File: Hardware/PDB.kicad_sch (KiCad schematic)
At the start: 52 parts, among them J1 Conn_01x02, J2 Conn_01x02, J3 Conn_01x02, J4 Conn_01x02, J5 Conn_01x02, Q1 Q_PMOS_GDS, U1 TPS54302, U2 TPS54302, U3 AP2112K-1.8, U4 INA219AxD

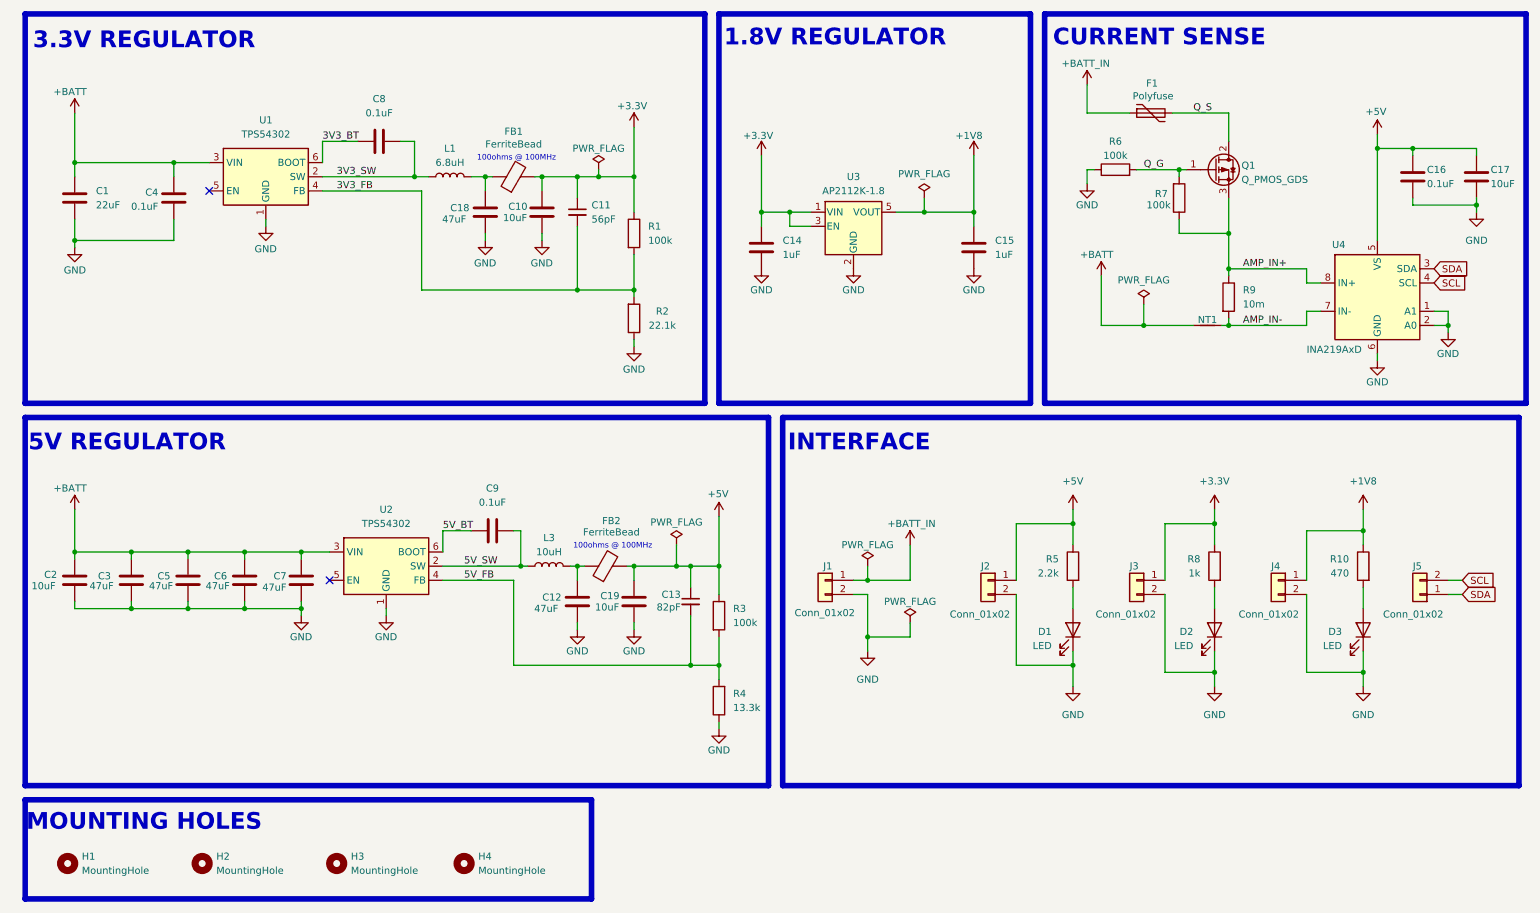
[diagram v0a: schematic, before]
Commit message: More changes
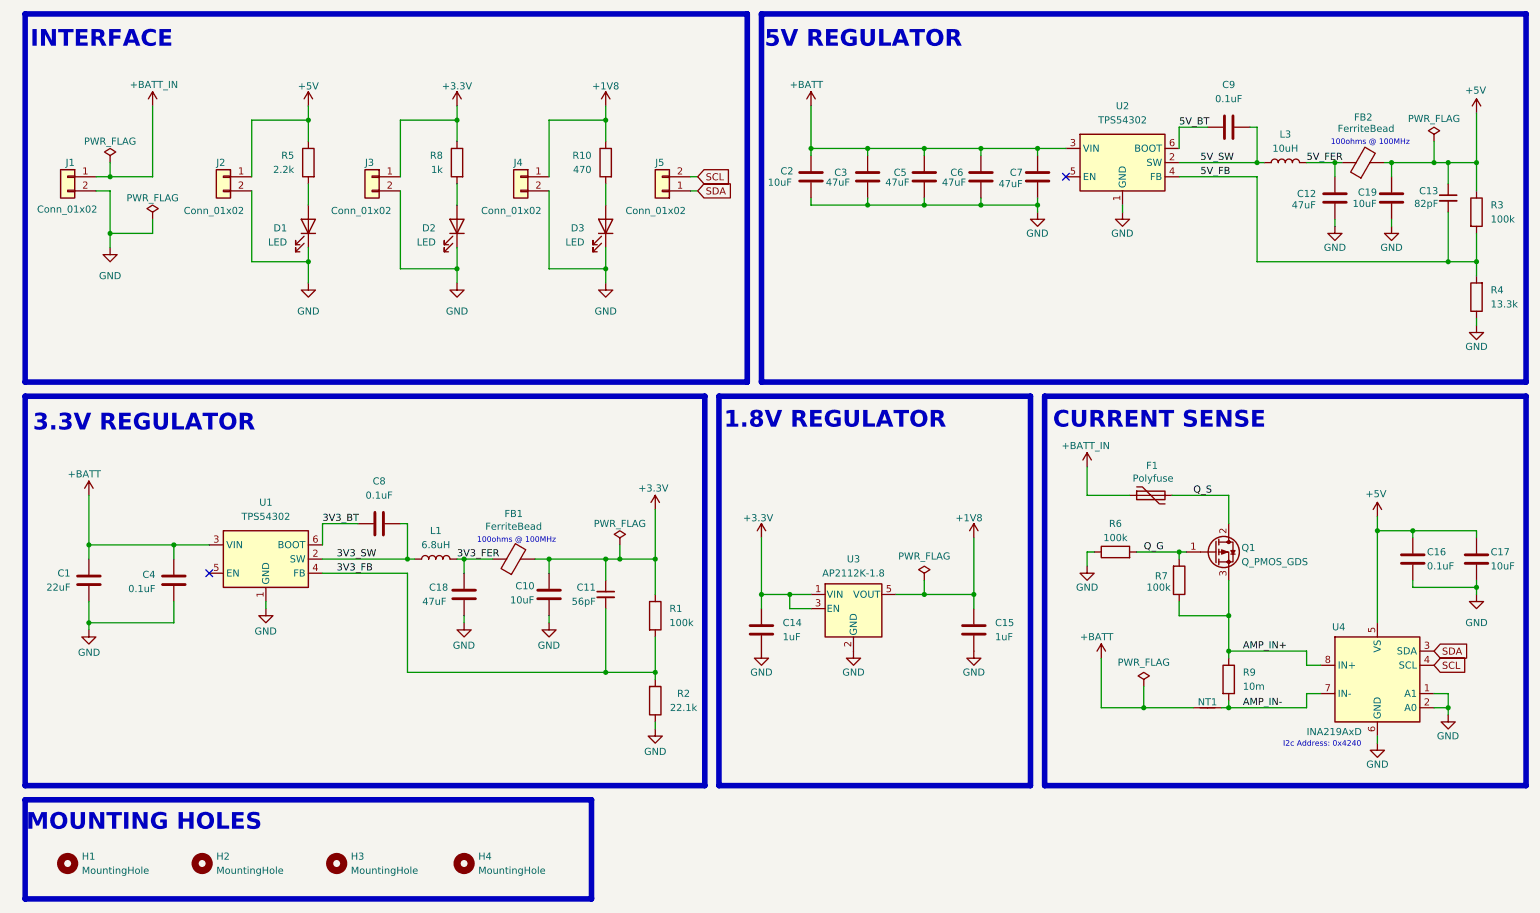
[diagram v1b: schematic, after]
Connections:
- net 5V_FER: now reaches C12.1, FB2.1, L3.2
- net 3V3_FER: now reaches C18.1, FB1.1, L1.2
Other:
- note added: "I2c Address: 0x4240"
- moved on the sheet: C1, C10, C11, C12, C13, C14, C15, C16, C17, C18, C19, C2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
